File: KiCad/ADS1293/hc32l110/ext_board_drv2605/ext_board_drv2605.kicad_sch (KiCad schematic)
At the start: 16 parts, among them J0 Conn_01x02_Male, J11 Conn_01x01_Female, J12 Conn_01x01_Female, J13 Conn_01x01_Female, J21 Conn_01x01_Female, J22 Conn_01x01_Female, J23 Conn_01x01_Female, J31 Conn_01x01_Female, J32 Conn_01x01_Female, J41 Conn_01x01_Female, J42 Conn_01x01_Female, J43 Conn_01x01_Female, M1 LRA, U1 DRV2605L, U2 WS2812-2020

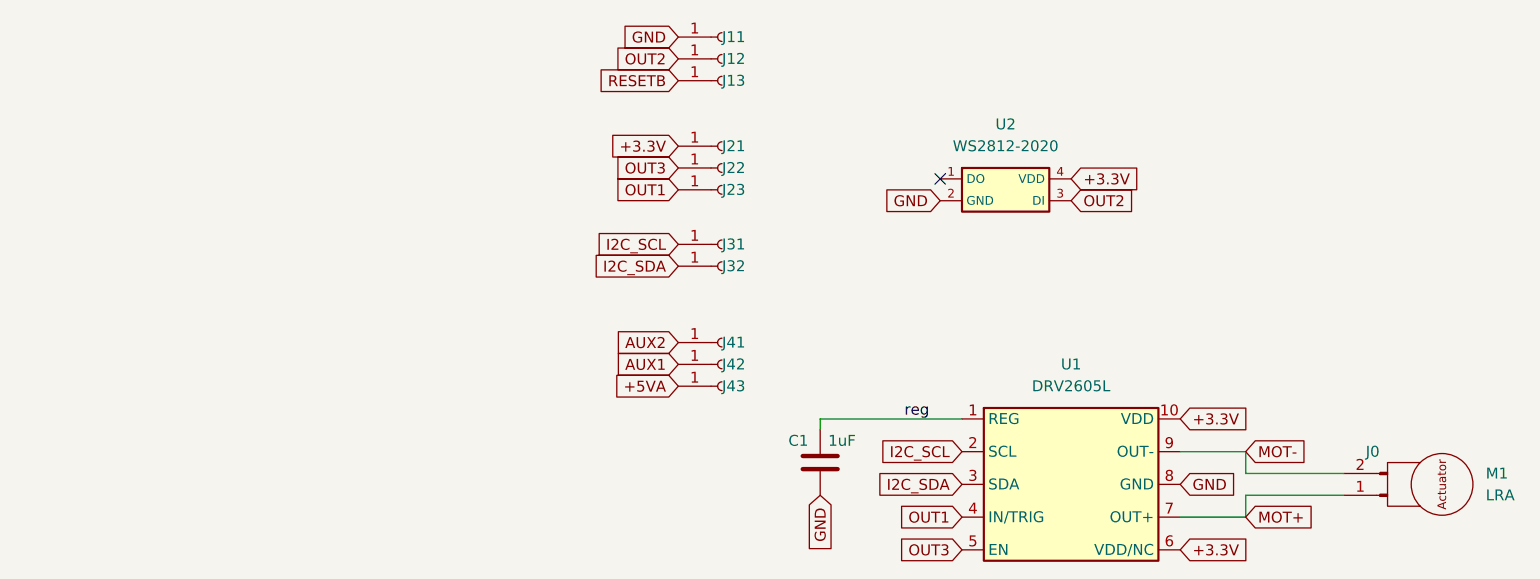
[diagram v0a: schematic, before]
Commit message: updated
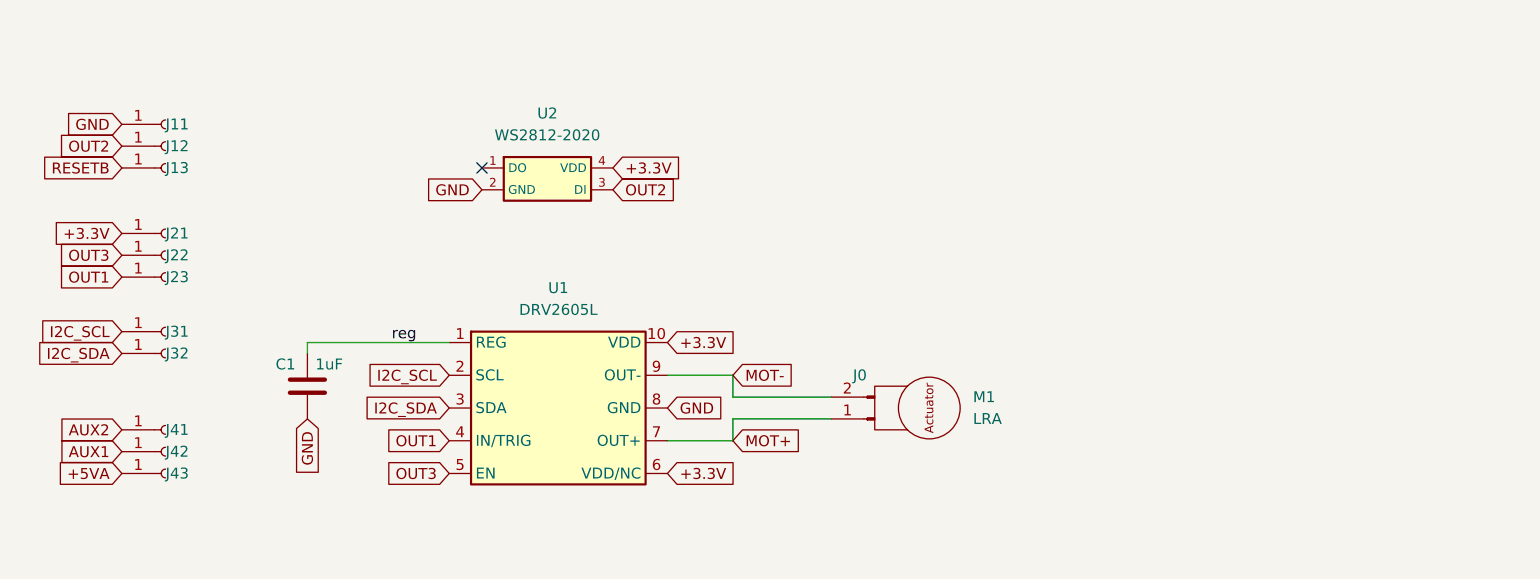
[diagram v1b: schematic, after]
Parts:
- M1: footprint 00_Custom:LRA0832BE03L15 -> 00_custom-footprints:LRA0832BE03L15
- U1: footprint 00_Custom:DRV2605L-VSSOP -> 00_custom-footprints:DRV2605L-VSSOP
- U2: footprint 00_Custom:WS2812-2020 -> 00_custom-footprints:WS2812-2020
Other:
- moved on the sheet: C1, J0, J11, J12, J13, J21, J22, J23, J31, J32, J41, J42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
